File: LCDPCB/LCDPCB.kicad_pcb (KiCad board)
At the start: 2 copper layers, 27 parts, among them J1 Sockets, J2 Hot Plug, J2 Hot plug, J3 Programming Header, J4 Conn_01x08_Male, J5 Conn_01x08_Male, SW1 SW_Push, U1 STM32F091RCT6, U2 LD1117S12TR_SOT223

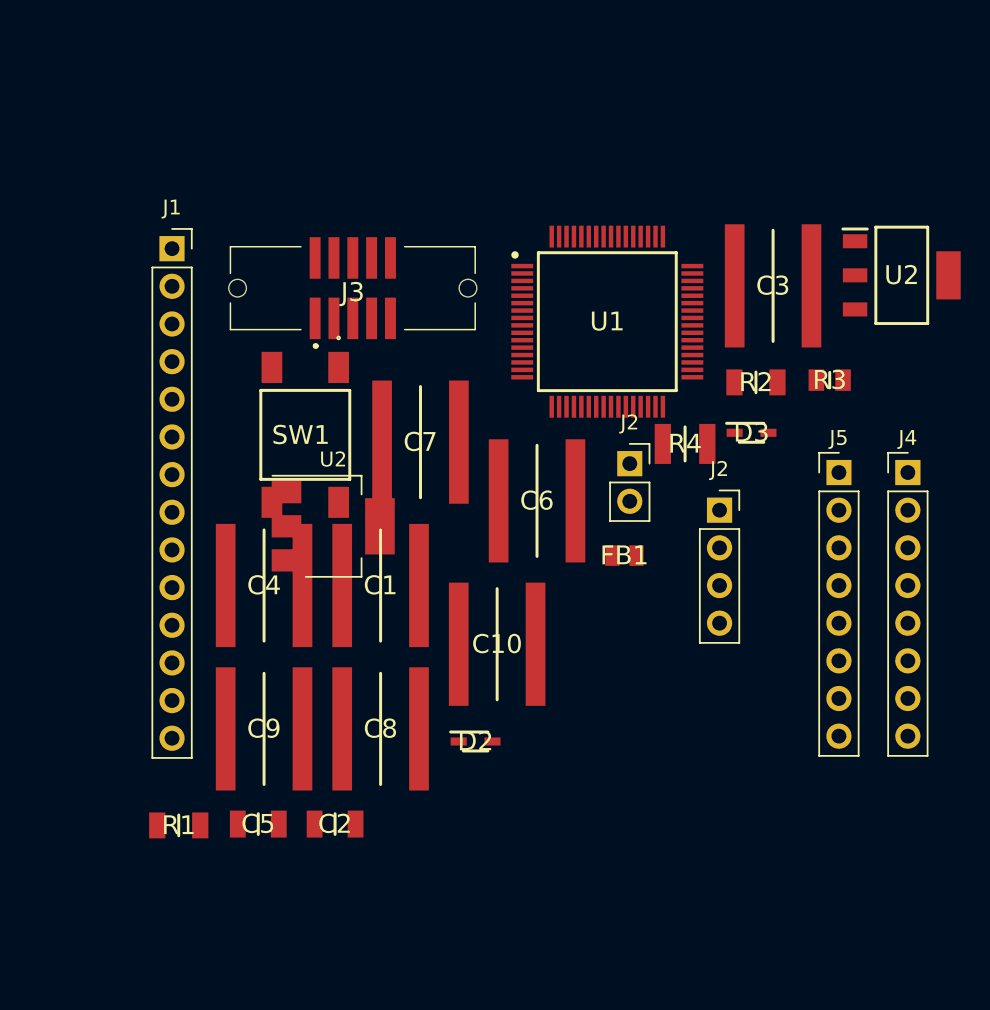
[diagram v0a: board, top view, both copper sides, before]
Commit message: display done
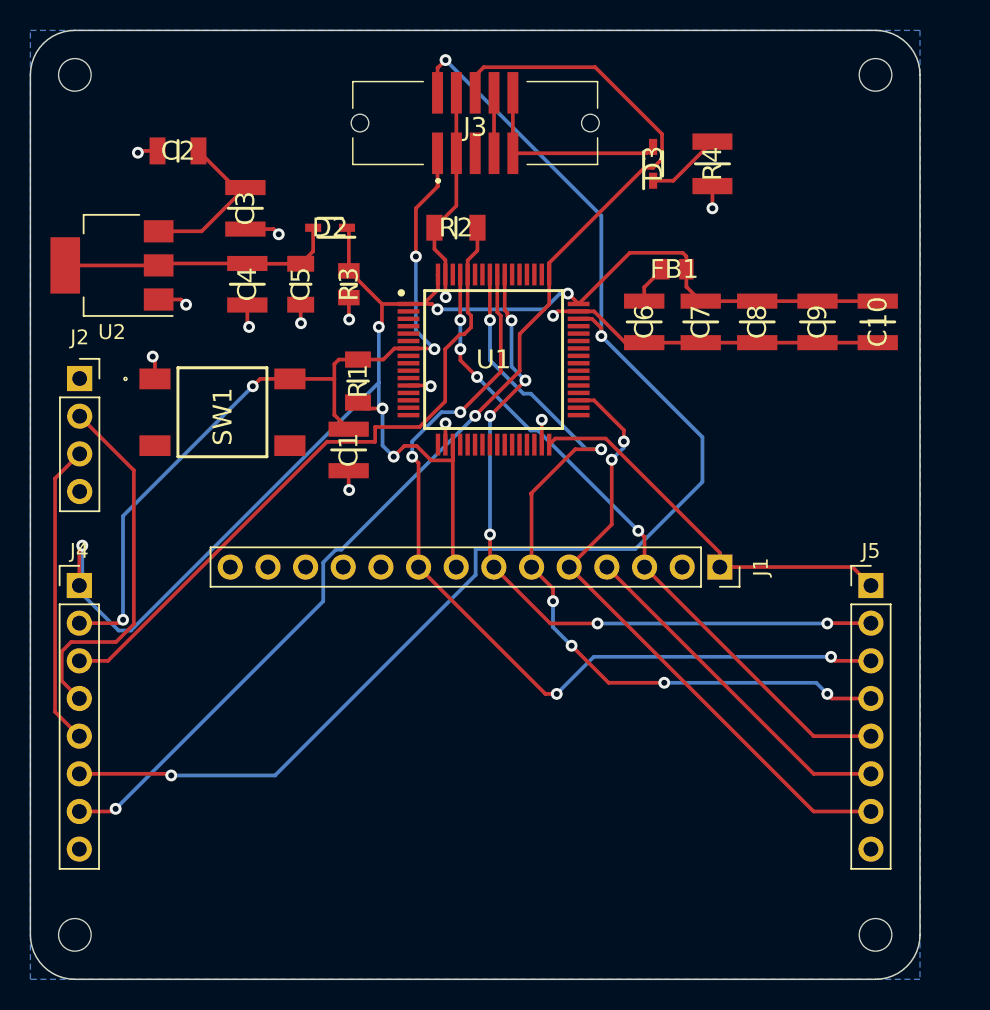
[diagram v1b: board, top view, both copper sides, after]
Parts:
- removed the J2 at (151.4, 83.2)
- removed the J2 at (157.5, 86.4)
- removed the U2 at (131.4, 87.4)
- removed the U2 at (169.8, 70.5)
- added H1: MountingHole, MountingHole:MountingHole_2.2mm_M2_ISO7380, F.Cu at (168.0, 57.0)
- added H2: MountingHole, MountingHole:MountingHole_2.2mm_M2_ISO7380, F.Cu at (168.0, 115.0)
- added H3: MountingHole, MountingHole:MountingHole_2.2mm_M2_ISO7380, F.Cu at (114.0, 57.0)
- added H4: MountingHole, MountingHole:MountingHole_2.2mm_M2_ISO7380, F.Cu at (114.0, 115.0)
- added J2: Hot Plug, Connector_PinSocket_2.54mm:PinSocket_1x04_P2.54mm_Vertical, F.Cu at (114.3, 77.5)
- added U2: LD1117S12TR_SOT223, Package_TO_SOT_SMD:SOT-223-3_TabPin2, F.Cu at (116.5, 69.8)
- C1, C10, C3, C4, C6, C7, C8, C9: footprint lib_file:.1uFC -> lib_file:CAPC3225X88N
- moved J4 56.4 mm to (114.3, 91.4)
- moved C2 46.6 mm to (121.0, 62.1), turned to 180 degrees
- moved C9 46.3 mm to (164.1, 73.7), turned to -90 degrees
- moved J1 42.7 mm to (157.5, 90.2), turned to -90 degrees
- moved C8 37.4 mm to (160.0, 73.7), turned to -90 degrees
- moved C5 36.5 mm to (129.2, 71.1), turned to -90 degrees
- moved D2 36.0 mm to (131.2, 67.3), turned to 180 degrees
- moved C3 36.0 mm to (125.5, 66.0), turned to -90 degrees
- moved C10 33.6 mm to (168.1, 73.7), turned to -90 degrees
- moved R3 33.1 mm to (132.5, 71.1), turned to -90 degrees
- moved R1 32.3 mm to (133.1, 77.7), turned to 90 degrees
- moved R2 22.8 mm to (139.7, 67.3)
- moved C7 20.6 mm to (156.2, 73.7), turned to -90 degrees
- moved C4 20.4 mm to (125.6, 71.1), turned to -90 degrees
- moved FB1 19.6 mm to (154.4, 70.1), turned to 180 degrees
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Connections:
- C10 pad 1: Net-(C10-Pad1) -> +3V0
- C7 pad 1: Net-(C10-Pad1) -> +3V0
- C8 pad 1: Net-(C10-Pad1) -> +3V0
- C9 pad 1: Net-(C10-Pad1) -> +3V0
- FB1 pad 1: Net-(C10-Pad1) -> +3V0
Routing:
- net +3V0: track 0.00 -> 134.1 mm, vias 0 -> 6
- net PA13: track 0.00 -> 91.7 mm, vias 0 -> 3
- net PA14: track 0.00 -> 79.7 mm, vias 0 -> 2
- net PB4: track 0.00 -> 58.4 mm, vias 0 -> 4
- net GND: track 0.00 -> 56.7 mm, vias 0 -> 14
- net PB5: track 0.00 -> 54.8 mm, vias 0 -> 6
- net NRST: track 0.00 -> 54.5 mm, vias 0 -> 4
- net PB3: track 0.00 -> 48.4 mm, vias 0 -> 6
- net PF11: track 0.00 -> 45.5 mm
- net PB8: track 0.00 -> 45.3 mm, vias 0 -> 4
- net PB14: track 0.00 -> 41.8 mm, vias 0 -> 2
- net PA6: track 0.00 -> 24.8 mm
- net PB11: track 0.00 -> 23.6 mm
- net PA7: track 0.00 -> 20.4 mm
- net Net-(C4-Pad1): track 0.00 -> 18.7 mm
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- added copper zone on B.Cu, net GND
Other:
- board outline added: 60 x 64 mm

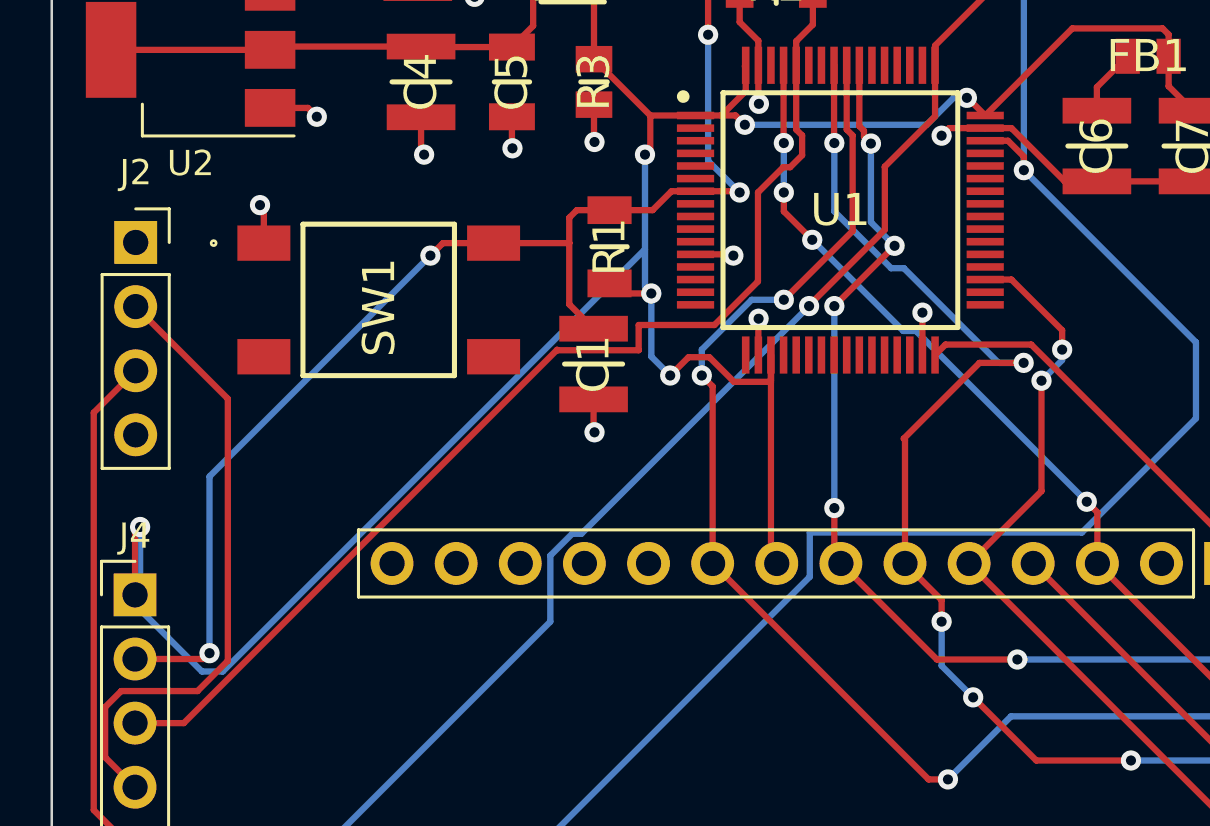
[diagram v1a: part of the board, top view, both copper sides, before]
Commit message: design mk 2
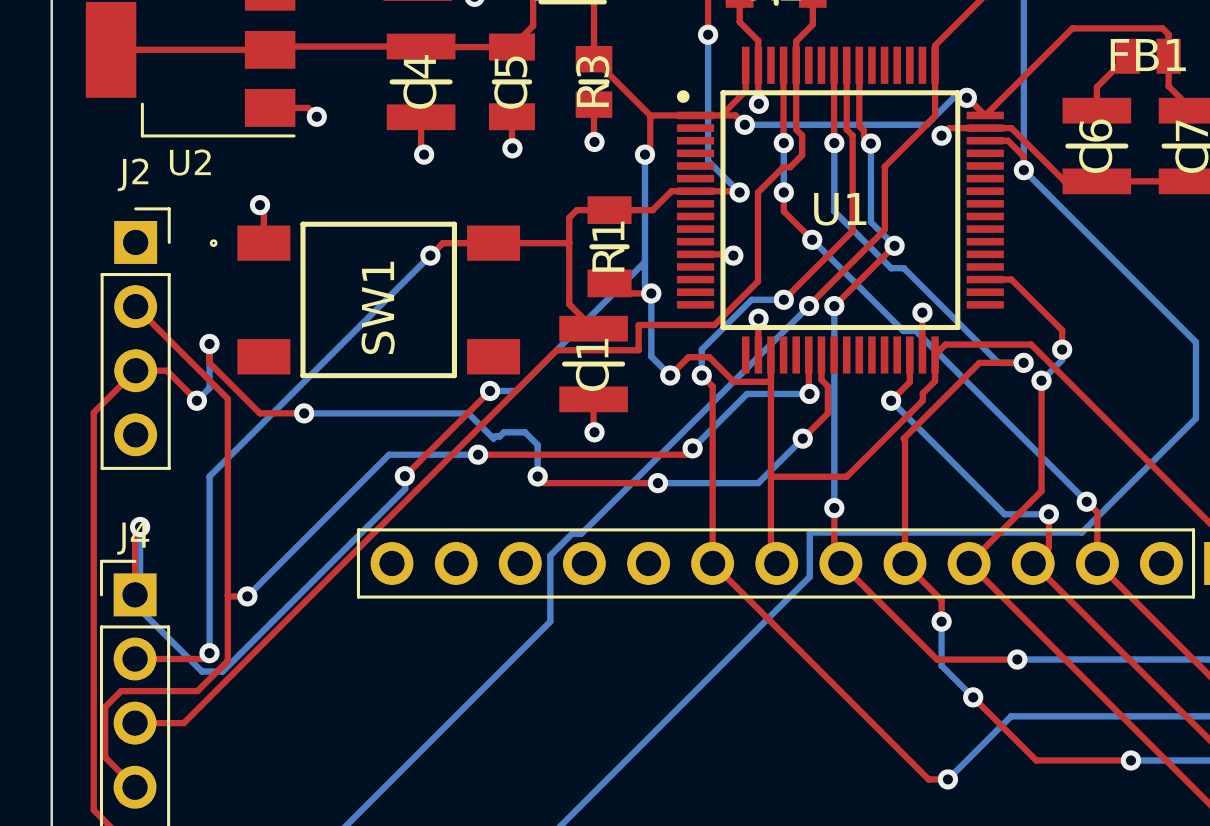
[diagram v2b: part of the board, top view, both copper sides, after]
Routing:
- net PA7: track 20.4 -> 57.5 mm, vias 0 -> 6
- net PA6: track 24.8 -> 52.8 mm, vias 0 -> 4
- net PB11: track 23.6 -> 36.0 mm, vias 0 -> 2
- net +3V0: track 134.1 -> 143.5 mm, vias 6 -> 8
